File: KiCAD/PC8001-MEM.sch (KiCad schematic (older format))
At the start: 29 parts, among them J1 PC-8001 ext BUS, U1 74LS32, U10 628128, U2 74LS138, U3 ULN2003A, U4 74LS138, U5 74LS175, U6 74LS32, U7 74LS541, U8 74LS273, U9 74LS541

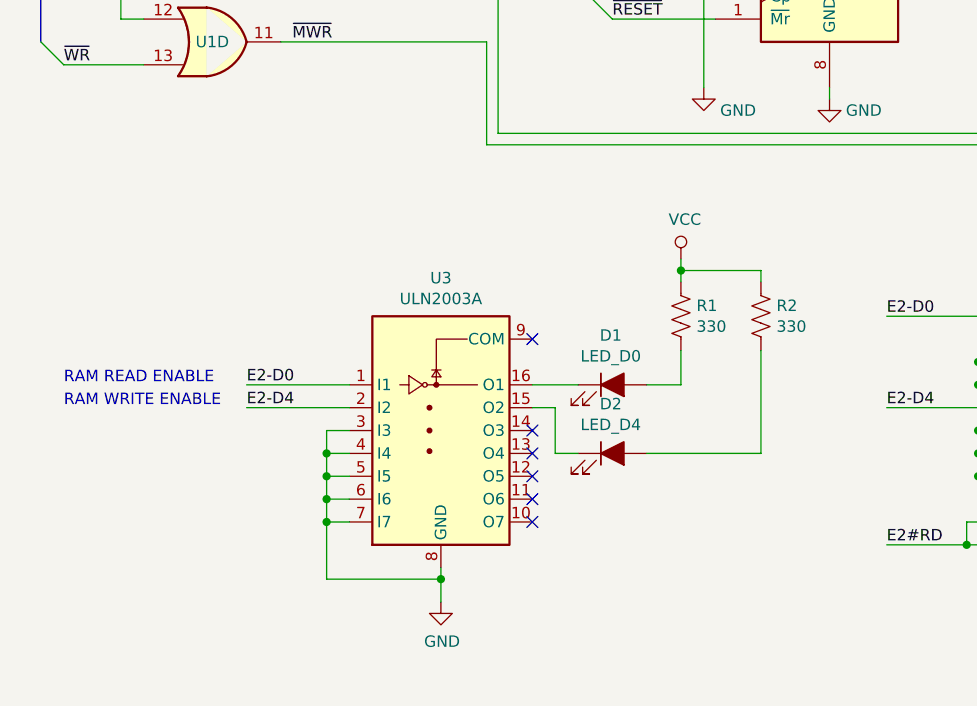
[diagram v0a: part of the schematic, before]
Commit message: プリント基板化検討
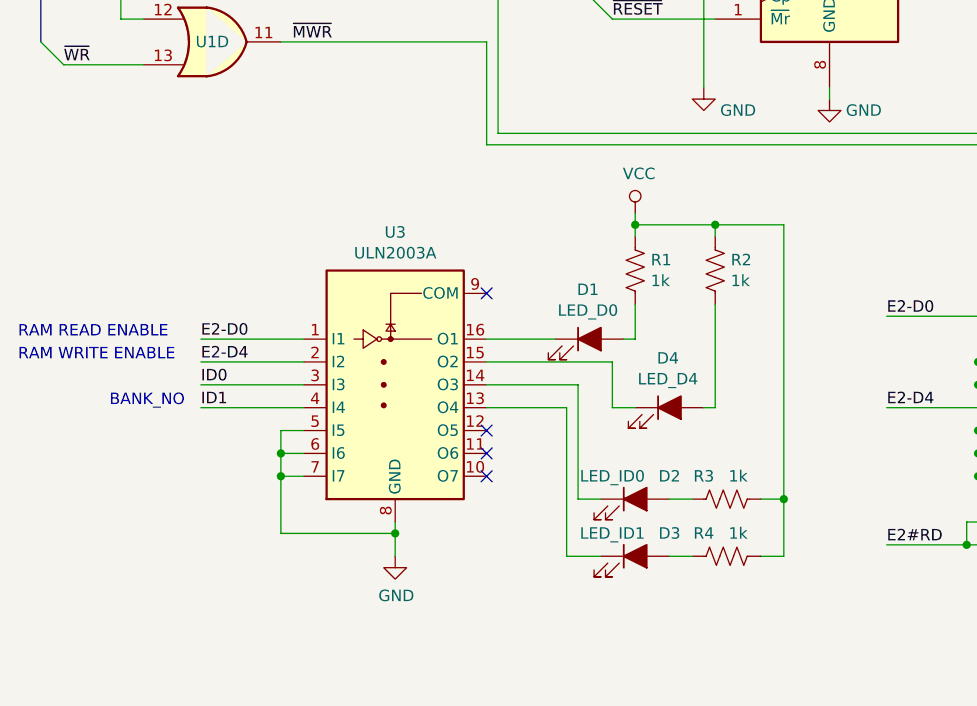
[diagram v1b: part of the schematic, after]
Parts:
- added D2: LED_ID0, LED_THT:LED_D3.0mm, symbol Device:LED_ALT
- added D3: LED_ID1, LED_THT:LED_D3.0mm, symbol Device:LED_ALT
- added R3, R4: 1k, Resistor_THT:R_Axial_DIN0207_L6.3mm_D2.5mm_P10.16mm_Horizontal, symbol Device:R_US
- C9: footprint (none) -> Capacitor_THT:CP_Radial_D5.0mm_P2.50mm
- D1: footprint (none) -> LED_THT:LED_D3.0mm
- D4: renamed from D2; footprint (none) -> LED_THT:LED_D3.0mm
- J1: footprint (none) -> Connector_PinHeader_2.54mm:PinHeader_2x25_P2.54mm_Horizontal
- R1, R2: value 330 -> 1k; footprint (none) -> Resistor_THT:R_Axial_DIN0207_L6.3mm_D2.5mm_P10.16mm_Horizontal
- U1, U6: footprint (none) -> Package_DIP:DIP-14_W7.62mm_Socket
- U10: footprint (none) -> Package_DIP:DIP-32_W15.24mm_Socket
- U2, U3, U4, U5: footprint (none) -> Package_DIP:DIP-16_W7.62mm_Socket
- U7, U8, U9: footprint (none) -> Package_DIP:DIP-20_W7.62mm_Socket
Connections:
- net GND: no longer U3.3 (I3), U3.4 (I4)
- net ID0: now also U3.3 (I3)
- net ID1: now also U3.4 (I4)
- net VCC: now also R3.1, R4.1
- net at U3.13 (O4): now also D3.1 (K)
- net at U3.14 (O3): now also D2.1 (K)
- new net: D2.2 (A), R3.2
- new net: D3.2 (A), R4.2
- no-connect marks 37 -> 35
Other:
- note added: "BANK_NO"
- moved on the sheet: D1, D4, R1, R2, U3
